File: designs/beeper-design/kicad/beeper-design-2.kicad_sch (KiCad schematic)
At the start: 37 parts, among them U12 DRV2605YZFR, U14 EVPBB4A9B000, U15 EVPBB4A9B000, U16 EVPBB4A9B000, U4 DA7212-01UM2, U5 FH19C-6S-0.5SH(10), U6 23-23B/R6GHBHW-C30/2A, U9 LSM6DSOXTR

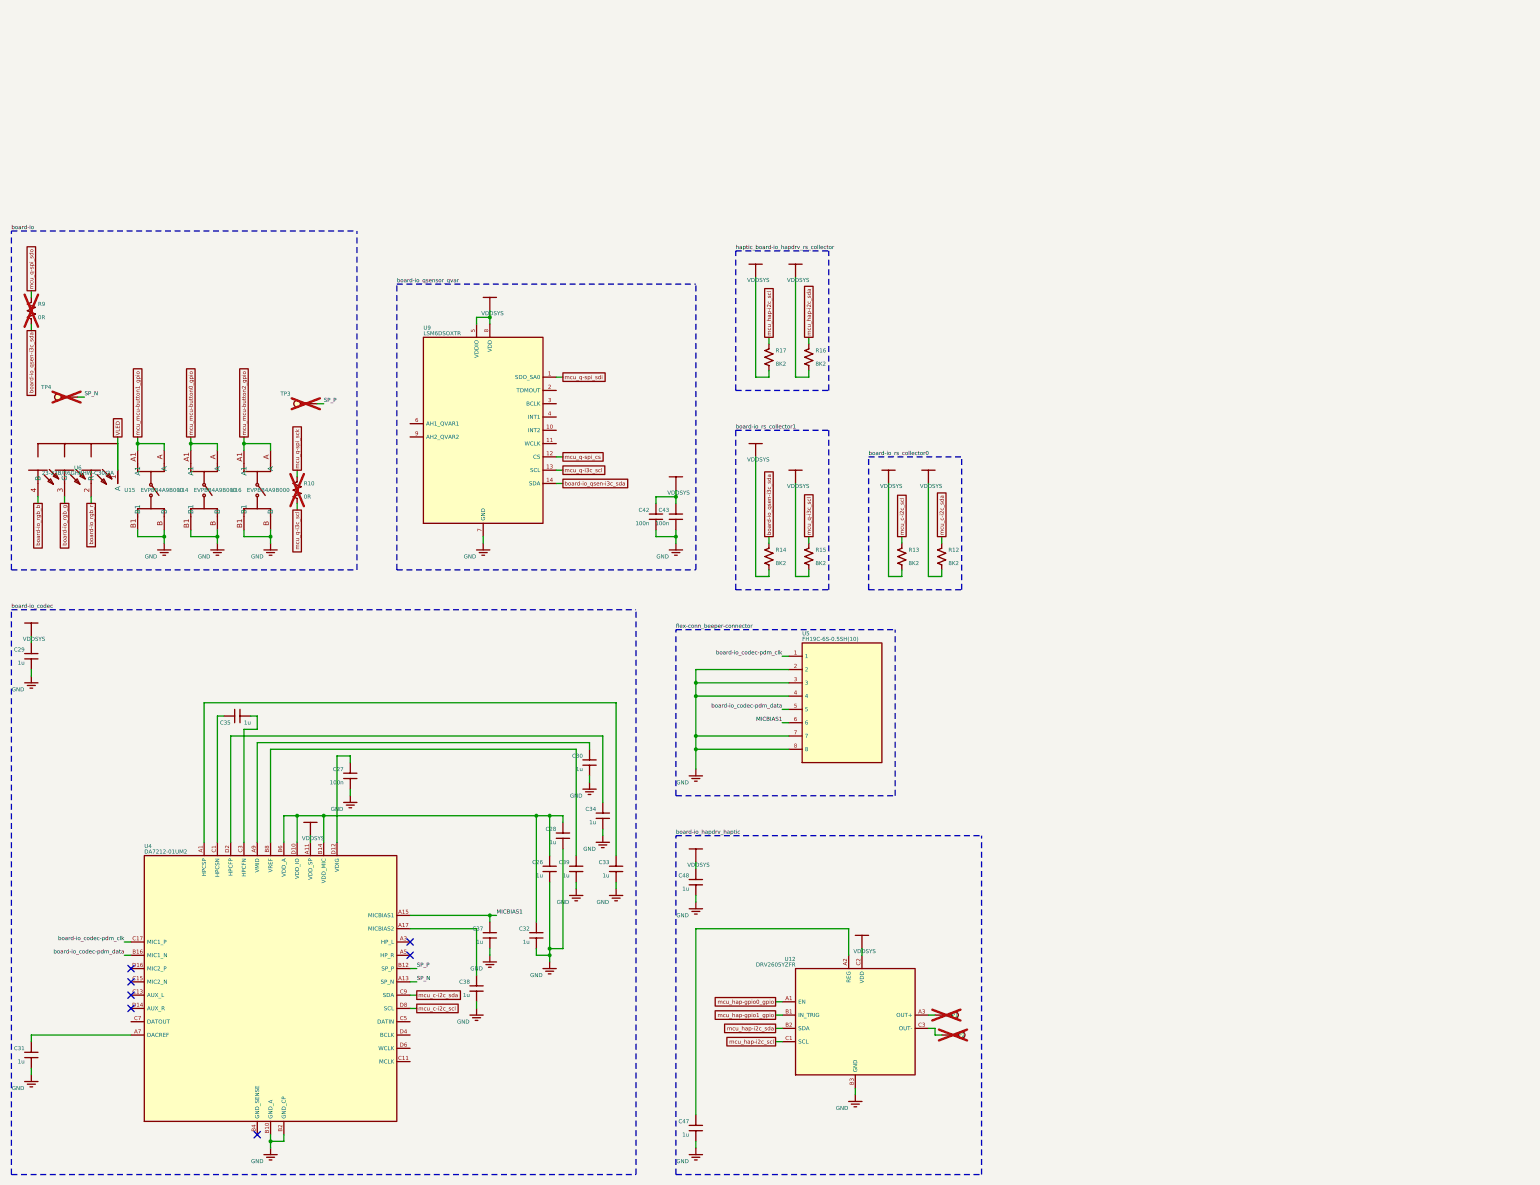
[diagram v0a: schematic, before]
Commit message: post export, had to munge sch
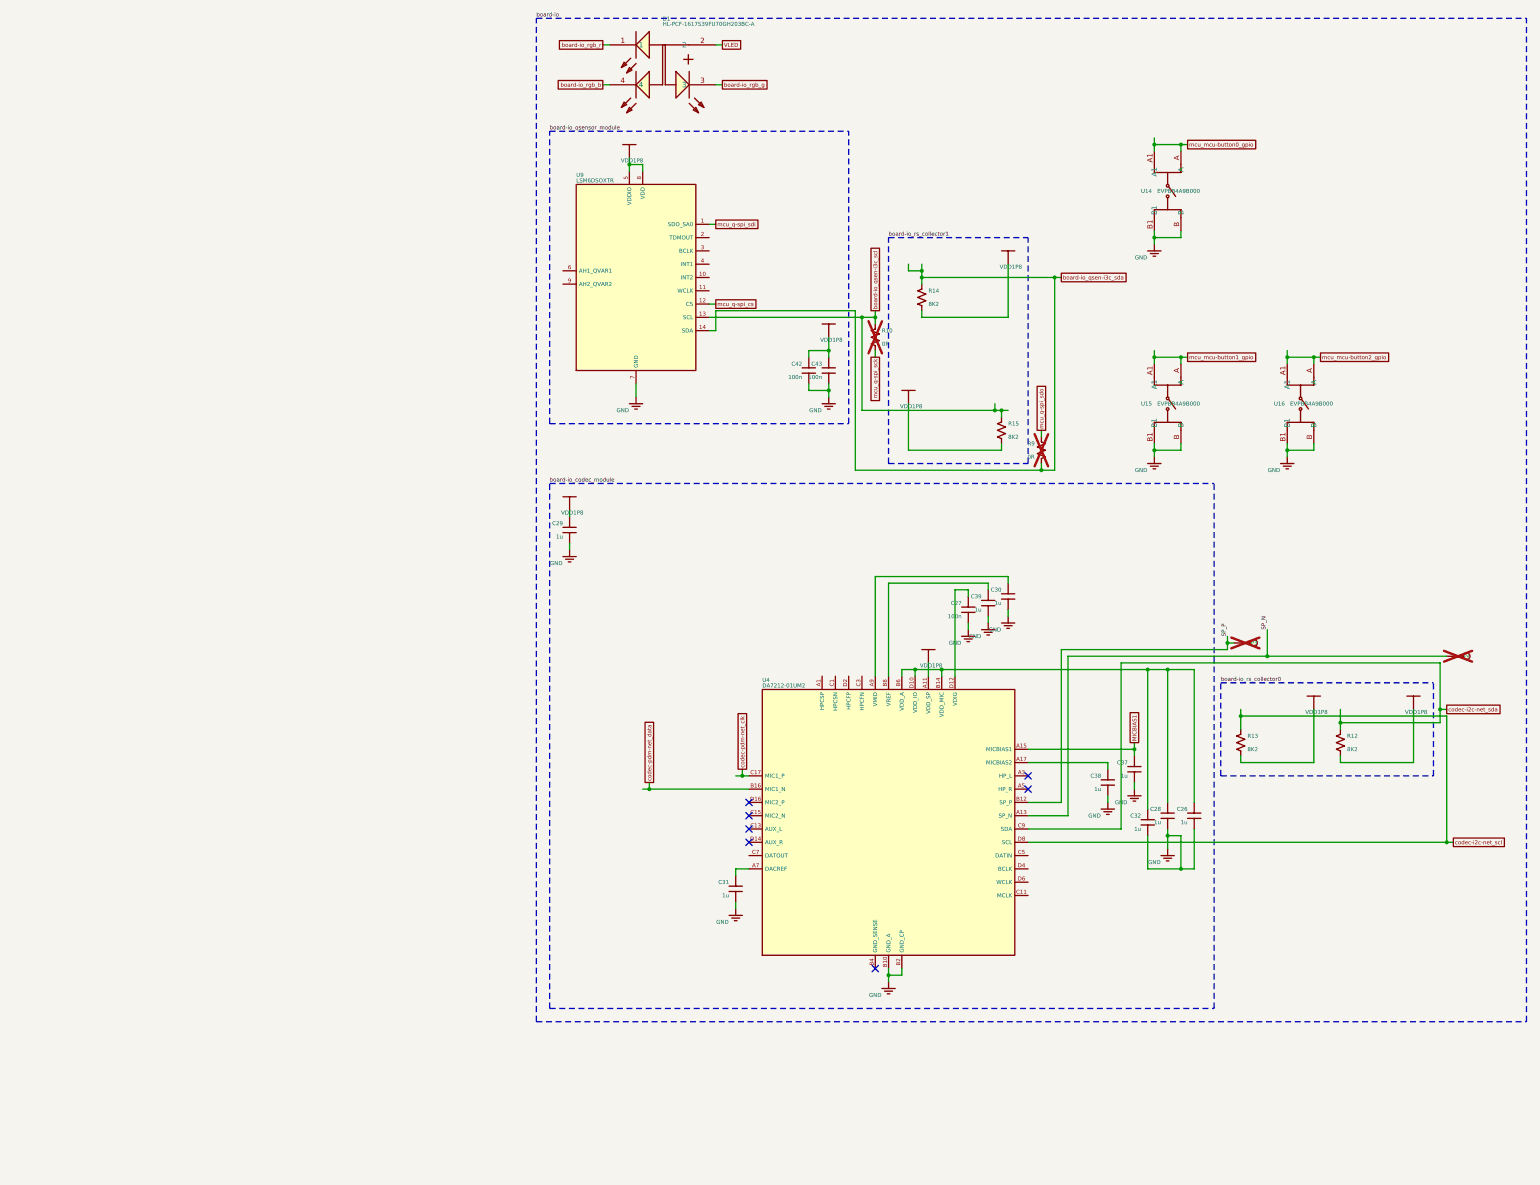
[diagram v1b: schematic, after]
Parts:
- removed C26: 1u, beeper-design:Pkg0201_37, symbol C76935_11
- removed C27: 100n, beeper-design:Pkg0201_44, symbol my_capacitor_7
- removed C28: 1u, beeper-design:Pkg0201_10, symbol C76935_2
- removed C29: 1u, beeper-design:Pkg0201_22, symbol C76935_6
- removed C30: 1u, beeper-design:Pkg0201_8, symbol C76935_1
- removed C31: 1u, beeper-design:Pkg0201_21, symbol C76935_5
- removed C32: 1u, beeper-design:Pkg0201_33, symbol C76935_9
- removed C33: 1u, beeper-design:Pkg0201_42, symbol C76935_12
- removed C34: 1u, beeper-design:Pkg0201_7, symbol C76935
- removed C35: 1u, beeper-design:Pkg0201_31, symbol C76935_8
- removed C37: 1u, beeper-design:Pkg0201_35, symbol C76935_10
- removed C38: 1u, beeper-design:Pkg0201_43, symbol C76935_13
- removed C39: 1u, beeper-design:Pkg0201_19, symbol C76935_4
- removed C42: 100n, beeper-design:Pkg0201_38, symbol my_capacitor_6
- removed C43: 100n, beeper-design:Pkg0201_1, symbol my_capacitor_9
- removed C47: 1u, beeper-design:Pkg0201_3, symbol C76935_14
- removed C48: 1u, beeper-design:Pkg0201_15, symbol C76935_3
- removed R10: 0R, beeper-design:Pkg0201_34, symbol C106228_2
- removed R12, R13: 8K2, beeper-design:Pkg0201_20, symbol my_resistor_2
- removed R16, R17: 8K2, beeper-design:Pkg0201_30, symbol my_resistor_3
- removed R9: 0R, beeper-design:Pkg0201_25, symbol C106228_1
- removed TP1, TP2: (no value), beeper-design:SMD_TESTPT, symbol smd_testpoint_cmp
- removed U12: DRV2605YZFR, beeper-design:LP_8, symbol DRV2605YZFR
- removed U5: FH19C-6S-0.5SH(10), beeper-design:LP_5, symbol FH19C_6S_0_5SH_10_
- added C26: 1u, beeper-design:Pkg0201_27, symbol C76935_8
- added C27: 100n, beeper-design:Pkg0201_38, symbol my_capacitor_13
- added C28: 1u, beeper-design:Pkg0201_5, symbol C76935_1
- added C29: 1u, beeper-design:Pkg0201_15, symbol C76935_5
- added C31: 1u, beeper-design:Pkg0201_13, symbol C76935_4
- added C32: 1u, beeper-design:Pkg0201_23, symbol C76935_6
- added C37: 1u, beeper-design:Pkg0201_26, symbol C76935_7
- added C38: 1u, beeper-design:Pkg0201_37, symbol C76935_10
- added C39: 1u, beeper-design:Pkg0201_35, symbol C76935_9
- added C42: 100n, beeper-design:Pkg0201_29, symbol my_capacitor_8
- added C43: 100n, beeper-design:Pkg0201_39, symbol my_capacitor_14
- added D1: HL-PCF-1617S39FU70GH203BC-A, beeper-design:LP_5, symbol C513368
- added R10: 0R, beeper-design:Pkg0201_28, symbol my_resistor_8
- added R12, R13: 8K2, beeper-design:Pkg0201_17, symbol my_resistor_4
- added TP3: (no value), beeper-design:SMD_TESTPT, symbol smd_testpoint_cmp
- C30: renamed from U6; value 23-23B/R6GHBHW-C30/2A -> 1u; footprint beeper-design:LP_4 -> beeper-design:Pkg0201_3; symbol L23_23B_R6GHBHW_C30_2A -> C76935; MPN 23-23B/R6GHBHW-C30/2A -> GRM033R61A105ME44D; Manufacturer Everlight -> MURATA; Name board-io_led -> board-io_codec_cap; Reference-prefix (none) -> C
- R14, R15: footprint beeper-design:Pkg0201_5 -> beeper-design:Pkg0201_1; MPN RC0201DR-078K2L -> RMCF0201JT8K20; Manufacturer YAGEO -> Stackpole Electronics Inc
- R9: renamed from TP3; value (none) -> 0R; footprint beeper-design:SMD_TESTPT -> beeper-design:Pkg0201_19; symbol smd_testpoint_cmp -> my_resistor_5; MPN (none) -> CR0201-J/-000GLF; Manufacturer (none) -> BOURNS; Name board-io_sp-pin0 -> board-io_rs-sda; Reference-prefix TP -> R
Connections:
- net GND: now also C30.1, C26.1, C27.1, C28.1, C29.1, C31.1, C32.1, C37.1, C38.1, C39.1, C42.1, C43.1
- net MICBIAS1: now also C37.2
- net SP_P: now also TP3.p; no longer R9.p
- net VLED: now also D1.2; no longer C30.1 (A)
- net board-io_qsen-i3c_sda: now also R9.1
- net board-io_rgb_b: now also D1.4; no longer C30.4 (B)
- net board-io_rgb_g: now also D1.3; no longer C30.3 (G)
- net board-io_rgb_r: now also D1.1; no longer C30.2 (R)
- net mcu_q-spi_sck: now also R10.2
- net mcu_q-spi_sdo: now also R9.2
- net at U4.A9 (VMID): now also C30.2
- net at U4.A17 (MICBIAS2): now also C38.2
- net at U4.A7 (DACREF): now also C31.2
- net at U4.B14 (VDD_MIC), U4.B6 (VDD_A), U4.D10 (VDD_IO): now also C26.2, C28.2, C32.2
- net at U4.B8 (VREF): now also C39.2
- net at U4.D12 (VDIG): now also C27.2
- net VDDSYS renamed VDD1P8
- net VDD1P8: now also C29.2, C42.2, C43.2, R12.2, R13.2
- net board-io_codec-pdm_clk renamed codec-pdm-net_clk
- net board-io_codec-pdm_data renamed codec-pdm-net_data
- net mcu_c-i2c_scl renamed codec-i2c-net_scl
- net codec-i2c-net_scl: now also R13.1
- net mcu_c-i2c_sda renamed codec-i2c-net_sda
- net codec-i2c-net_sda: now also R12.1
- net mcu_q-i3c_scl renamed board-io_qsen-i3c_scl
- net board-io_qsen-i3c_scl: now also R10.1
